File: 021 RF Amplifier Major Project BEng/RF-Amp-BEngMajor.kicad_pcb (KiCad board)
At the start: 4 copper layers, 28.6 x 49.5 mm, 62 parts, among them SW1 SW_SPDT, U1 THS4302RGTT

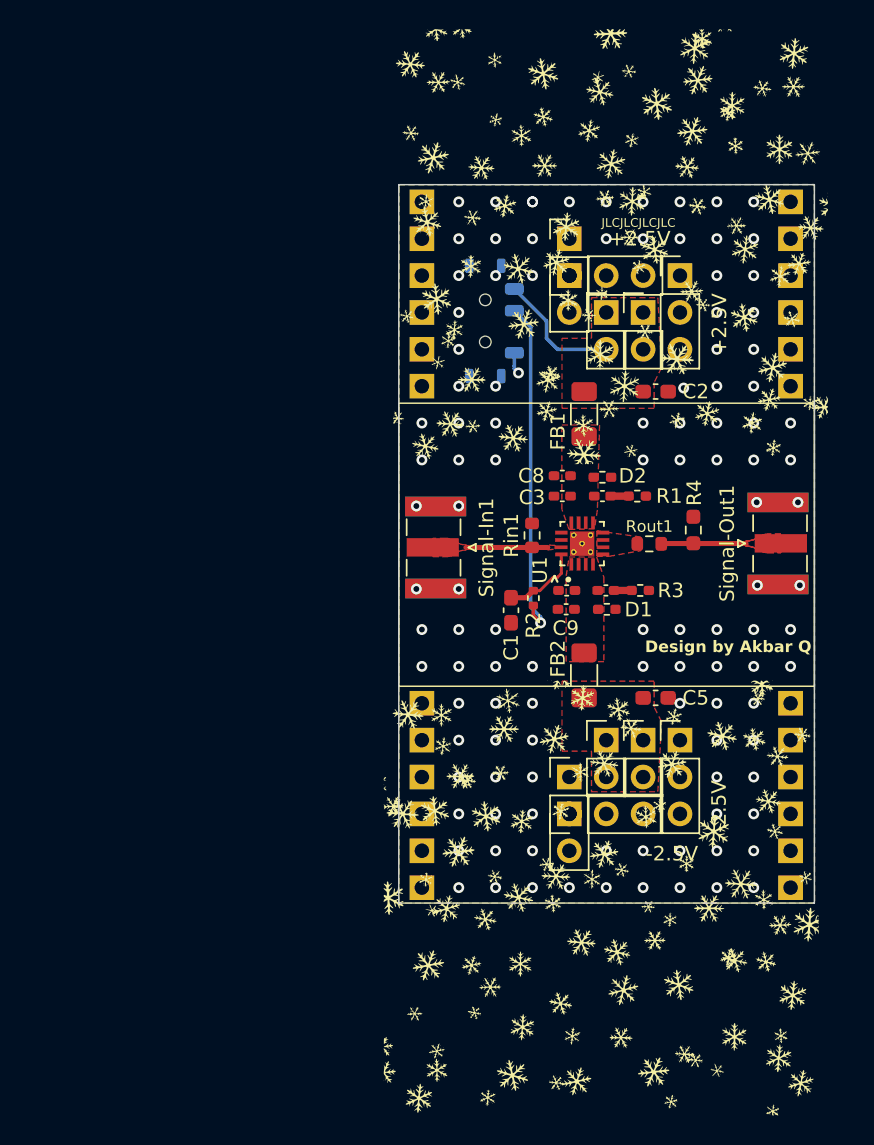
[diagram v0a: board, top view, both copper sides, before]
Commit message: Comments Modified
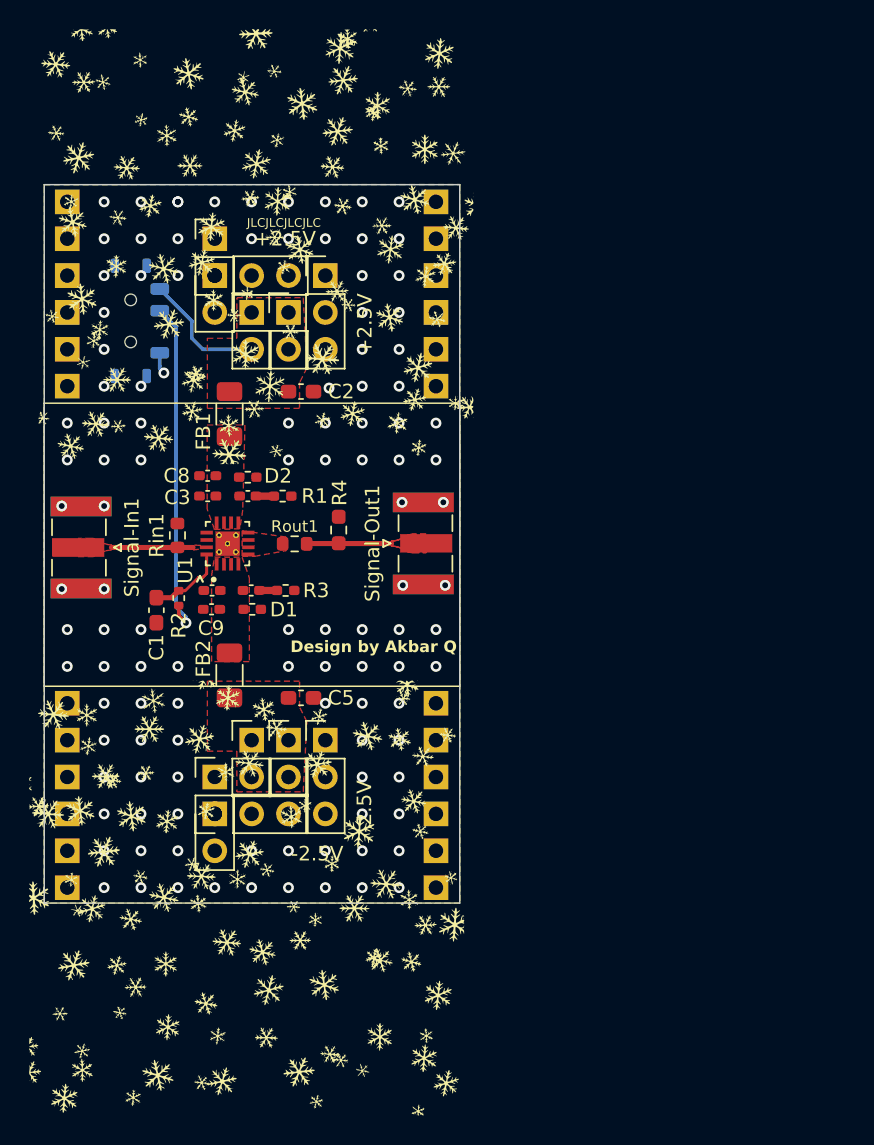
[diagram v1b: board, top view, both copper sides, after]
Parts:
- moved +G1 24.4 mm to (44.5, 34.6)
- moved -G3 24.4 mm to (44.5, 66.6)
- moved Signal-Out1 24.4 mm to (51.2, 53.1)
- moved +2.5V 24.4 mm to (41.9, 37.1)
- moved +2.5V 24.4 mm to (39.4, 37.1)
- moved +G2 24.4 mm to (36.9, 34.6)
- moved +G3 24.4 mm to (36.9, 32.1)
- moved -2.5V 24.4 mm to (39.4, 66.6)
- moved -2.5V 24.4 mm to (41.9, 66.6)
- moved -G1 24.4 mm to (36.9, 69.2)
- moved -G4 24.4 mm to (36.9, 71.7)
- moved C1 24.4 mm to (32.8, 57.7)
- moved C2 24.4 mm to (42.8, 42.6)
- moved C3 24.4 mm to (36.4, 49.8)
- moved C4 24.4 mm to (39.1, 49.8)
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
